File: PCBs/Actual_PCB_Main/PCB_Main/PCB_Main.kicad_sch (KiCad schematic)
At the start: 145 parts, among them J1 fan connector, J10 To_Speaker_R, J2 10118193-0001LF, J4 10118193-0001LF, J6 XT60-M, J7 HUB75, J9 To_Speaker_L, M1 CSD17581Q3, M2 CSD17581Q3A, Q1 S8050, Q2 S8050, Q4 Fan_NMOS, Q5 S8050, Q6 S8050, SW1 SW_Push, SW2 SW_Push, SW3 SW_Push, SW4 SW_Push, U1 CP2102N-Axx-xQFN28, U2 AMS1117-3.3, U3 ESP32-WROOM-E, U4 PCM5102A, U5 LM5122MH/NOPB, U6 ESP32-WROVER-E, U7 LM4752TS, U9 CP2102N-Axx-xQFN28, Y1 CB3LV-3I-40M000000, Y2 CB3LV-3I-40M000000

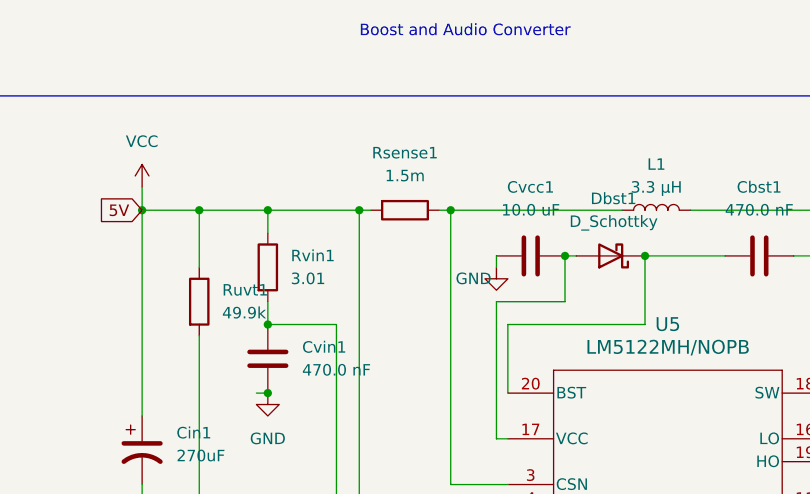
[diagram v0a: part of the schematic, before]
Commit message: PCB reset traces
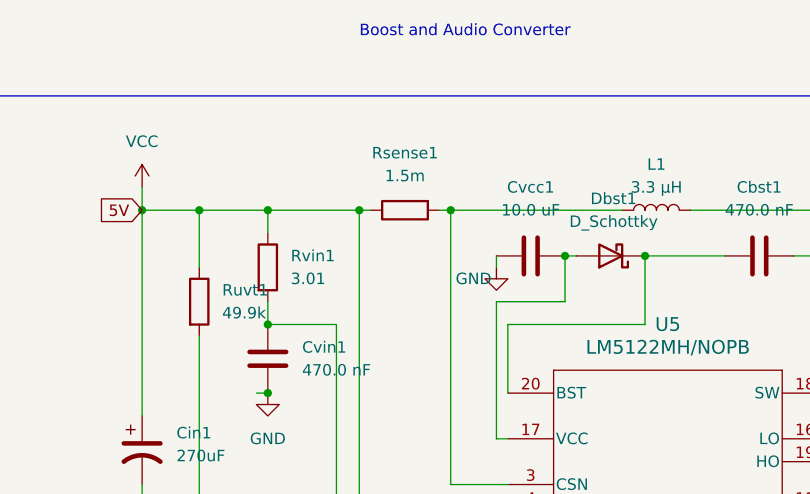
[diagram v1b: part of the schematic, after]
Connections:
- net VCC: now also Rsense1.1; no longer Rsense1.2
- net at L1.1, U5.3 (CSN): now also Rsense1.2; no longer Rsense1.1
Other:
- moved on the sheet: Rsense1
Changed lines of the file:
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@@
     )
   )
-  (symbol (lib_id "Device:R") (at 50.8 -74.93 270) (unit 1)
-    (in_bom yes) (on_board yes) (dnp no) (fields_autoplaced)
+  (symbol (lib_id "Device:R") (at 50.8 -74.93 90) (mirror x) (unit 1)
+    (in_bom yes) (on_board yes) (dnp no)
     (property "Reference" "Rsense1" (at 50.8 -81.28 90)
       (effects (font (size 1.27 1.27)))
@@
   )
   (symbol (lib_id "power:GND") (at 316.23 87.63 0) (unit 1)
-    (in_bom yes) (on_board yes) (dnp no) (fields_autoplaced)
+    (in_bom yes) (on_board yes) (dnp no)
     (property "Reference" "#PWR09" (at 316.23 93.98 0)
       (effects (font (size 1.27 1.27)) hide)
